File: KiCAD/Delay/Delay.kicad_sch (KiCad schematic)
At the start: 65 parts, among them J1 IN, J2 OUT, J3 Conn_01x03, J4 Conn_01x03, U1 TL072, U2 TL072, U3 PT2399, U4 L7805

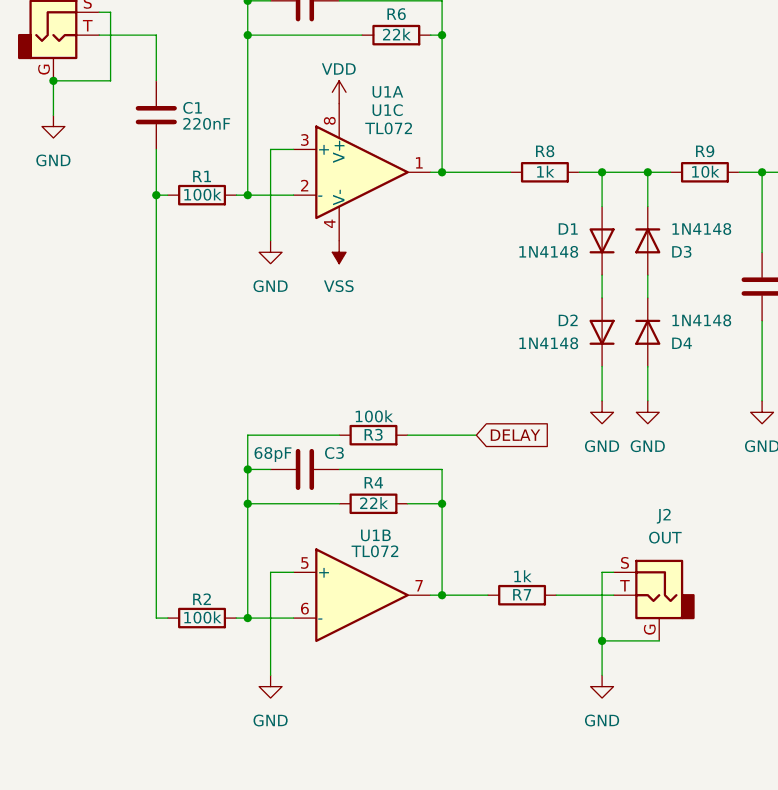
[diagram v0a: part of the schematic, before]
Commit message: Delay PCB
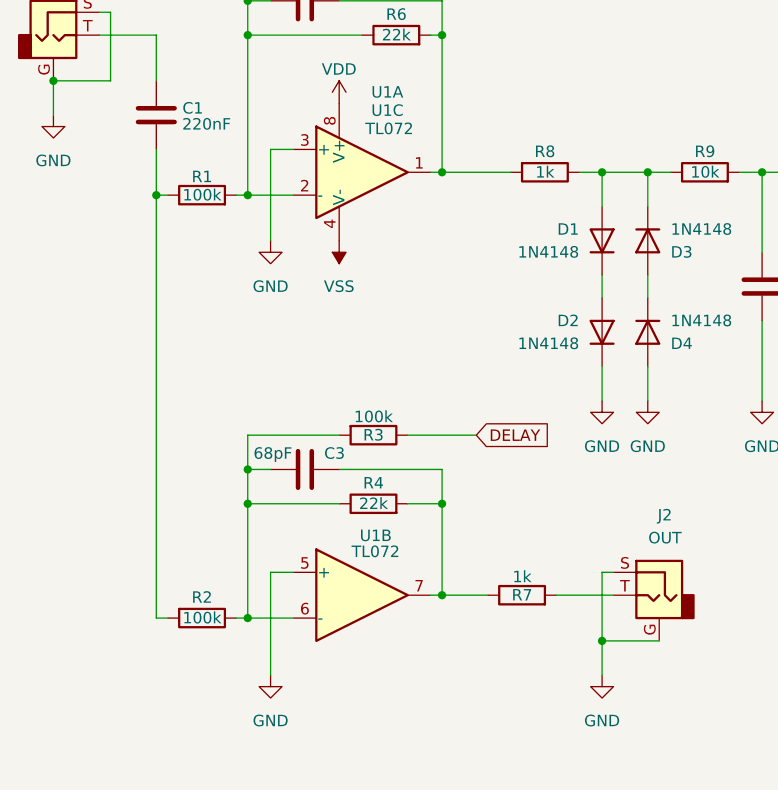
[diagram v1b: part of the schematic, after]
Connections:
- net DELAY: now also R3.1; no longer R3.2
- net at C2.1, R6.2, U1.1: now also R8.2; no longer R8.1
- net at C3.2, R4.1, U1.6 (-): now also R2.1, R3.2; no longer R2.2, R3.1
- net at D1.2 (A), D3.1 (K), R9.1: now also R8.1; no longer R8.2
- net at C1.1, R1.1: now also R2.2; no longer R2.1
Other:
- moved on the sheet: R2, R3, R8
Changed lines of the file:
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@@
 	(symbol
 		(lib_id "HackSynth:R")
-		(at 62.23 78.74 90)
+		(at 62.23 78.74 270)
 		(unit 1)
 		(exclude_from_sim no)
@@
 		)
 		(property "Footprint" "HackSynth:R_Vertical_P2.54mm"
-			(at 62.23 80.518 90)
+			(at 62.23 76.962 90)
 			(effects
 				(font
@@
 	(symbol
 		(lib_id "HackSynth:R")
-		(at 81.28 49.53 90)
+		(at 81.28 49.53 270)
 		(unit 1)
 		(exclude_from_sim no)
@@
 		)
 		(property "Footprint" "HackSynth:R_Vertical_P2.54mm"
-			(at 81.28 51.308 90)
+			(at 81.28 47.752 90)
 			(effects
 				(font
@@
 	(symbol
 		(lib_id "HackSynth:R")
-		(at 43.18 99.06 90)
+		(at 43.18 99.06 270)
 		(unit 1)
 		(exclude_from_sim no)
@@
 		(dnp no)
 		(property "Reference" "R2"
-			(at 43.18 97.028 90)
+			(at 43.18 96.774 90)
 			(effects
 				(font
@@
 		)
 		(property "Footprint" "HackSynth:R_Vertical_P2.54mm"
-			(at 43.18 100.838 90)
+			(at 43.18 97.282 90)
 			(effects
 				(font

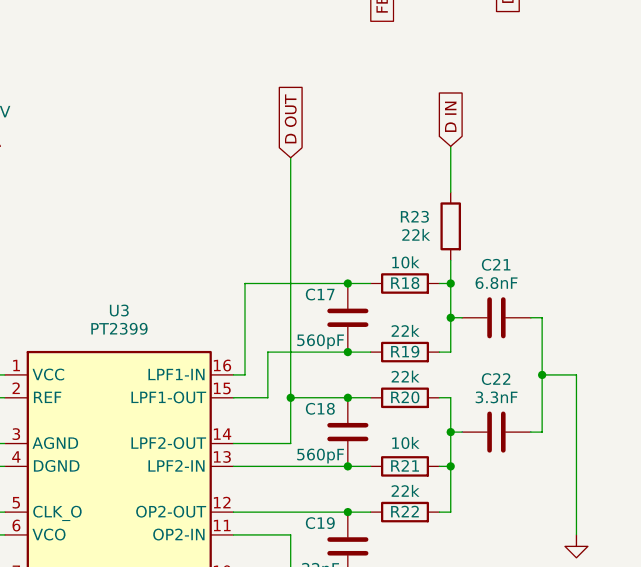
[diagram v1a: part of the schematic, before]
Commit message: Delay PCB
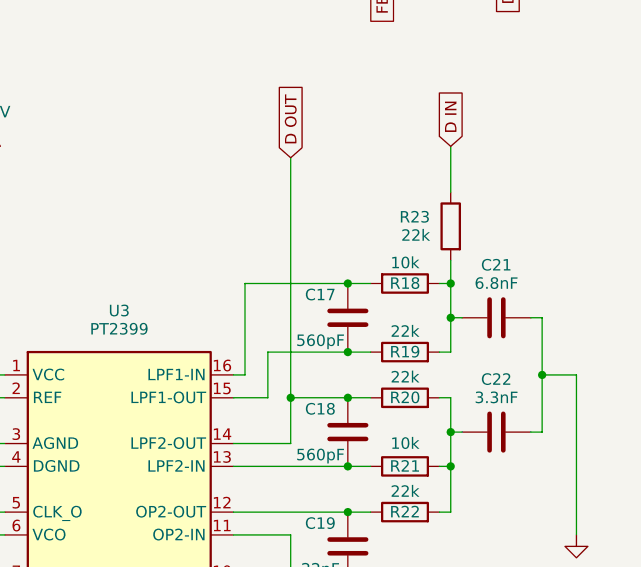
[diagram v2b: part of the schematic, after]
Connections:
- net at C21.2, R19.2, R23.2: now also R18.1; no longer R18.2
- net at C17.1, U3.16 (LPF1-IN): now also R18.2; no longer R18.1
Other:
- moved on the sheet: R18
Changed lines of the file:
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@@
 			"gtJqHJTWHJSWgtJqHJTWHJSWgtJqHJTWHJSWgtJqHJTWHJSWIpK2hxHREqNQWjNQWoq1tJcDEW2x"
 			"j38zCAGlpVhLiyAaBqWloLSIF/HOJ7z9UadpjtIi3kM6v9Ov2xhL/v/mElWvvu6fRQAAAABJRU5E"
-			"rkJggg=="
+			"rkJgggAgACAAIAAgACAAIAAgAD0AIAAiAHMAdABhAHQAaQBjAHQAZQB4AHQAIgANAA0ACgAvAD4A"
+			"DQANAAoAPAAvAGkAZgA+AA0ADQAKADwAaQBmACAAaQBkAD0AIgBhAHQAbwBtACgARgBvAG8AdABu"
+			"AG8AdABlAFQAZQB4AHQATABpAG4AawApACIAPgANAA0ACgA8AGMAYwBzAHkAcwBsAGkAbgBrAA0A"
+			"DQAKAGYAbwBuAHQAIAAgACAAIAAgACAAIAAgACAAIAAgACAAIAAgACAAIAA9ACAAIgBnAHQAZgAo"
+			"AFQAYQBzAGsARABpAGEAbABvAGcAUwB0AHkAbABlACwAIAAxADUALAAgADAAKQAiAA0ADQAKAGYA"
+			"bwByAGUAZwByAG8AdQBuAGQAIAAgACAAIAAgACAAIAAgACAAIAA9ACAAIgBnAHQAYwAoAFQAYQBz"
+			"AGsARABpAGEAbABvAGcAUwB0AHkAbABlACwAIAAxADUALAAgADAALAAgADMAOAAwADMAKQAiAA0A"
+			"DQAKAC8APgANAA0ACgA8AC8AaQBmAD4ADQANAAoAPABpAGYAIABpAGQAPQAiAGEAdABvAG0AKABF"
+			"AHgAcABhAG4AZABlAGQARgBvAG8AdABlAHIAQQByAGUAYQApACIAPgANAA0ACgA8AGUAbABlAG0A"
+			"ZQBuAHQADQANAAoAYgBhAGMAawBnAHIAbwB1AG4AZAAgACAAIAAgACAAIAAgACAAIAAgAD0AIAAi"
+			"AHQAaABlAG0AZQBhAGIAbABlACgAZAB0AGIAKABUAGEAcwBrAEQAaQBhAGwAbwBnACwAIAAxADUA"
+			"LAAgADAAKQAsACAAdABoAHIAZQBlAGQAZgBhAGMAZQApACIADQANAAoAcABhAGQAZABpAG4AZwAg"
+			"ACAAIAAgACAAIAAgACAAIAAgACAAIAAgAD0AIAAiAHQAaABlAG0AZQBhAGIAbABlACgAZwB0AG0A"
+			"YQByACgAVABhAHMAawBEAGkAYQBsAG8AZwAsACAAMQA4ACwAIAAwACwAIAAzADYAMAAyACkALABy"
+			"AGUAYwB0ACgAMQAwAHIAcAAsADAALAAxADAAcgBwACwANQByAHAAKQApACIADQANAAoALwA+AA0A"
+			"DQAKADwALwBpAGYAPgANAA0ACgA8AGkAZgAgAGkAZAA9ACIAYQB0AG8AbQAoAEUAeABwAGEAbgBk"
+			"AGUAZABGAG8AbwB0AGUAcgBUAGUAeAB0ACkAIgA+AA0ADQAKADwAZQBsAGUAbQBlAG4AdAANAA0A"
+			"CgBmAG8AbgB0ACAAIAAgACAAIAAgACAAIAAgACAAIAAgACAAIAAgACAAPQAgACIAZwB0AGYAKABU"
+			"AGEAcw=="
 		)
 	)
@@
 	(symbol
 		(lib_id "HackSynth:R")
-		(at 251.46 95.25 90)
+		(at 251.46 95.25 270)
 		(unit 1)
 		(exclude_from_sim no)
@@
 		)
 		(property "Footprint" "HackSynth:R_Vertical_P2.54mm"
-			(at 251.46 97.028 90)
+			(at 251.46 93.472 90)
 			(effects
 				(font
